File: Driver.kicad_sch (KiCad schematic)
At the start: 25 parts

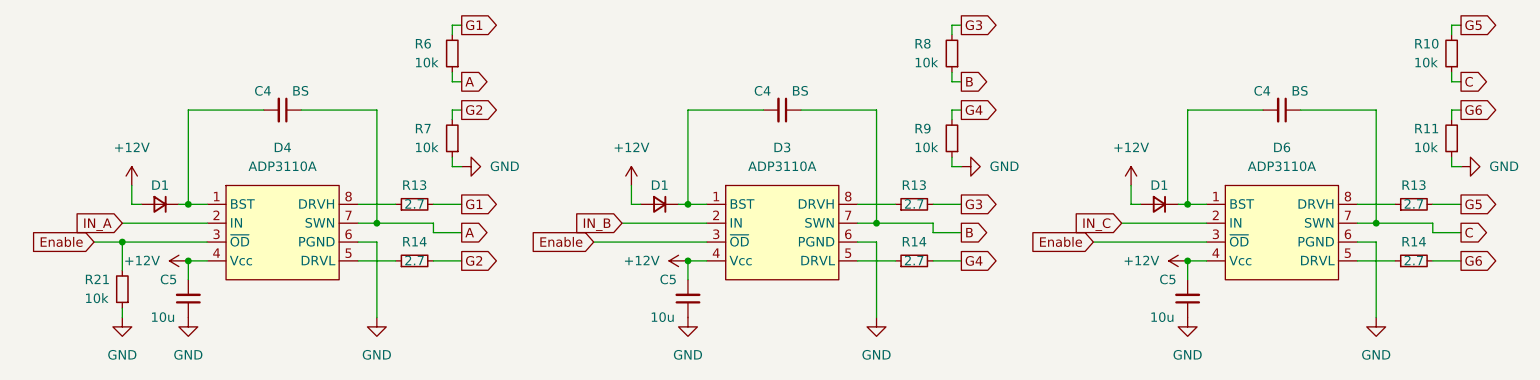
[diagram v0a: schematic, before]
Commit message: Стартовая версия
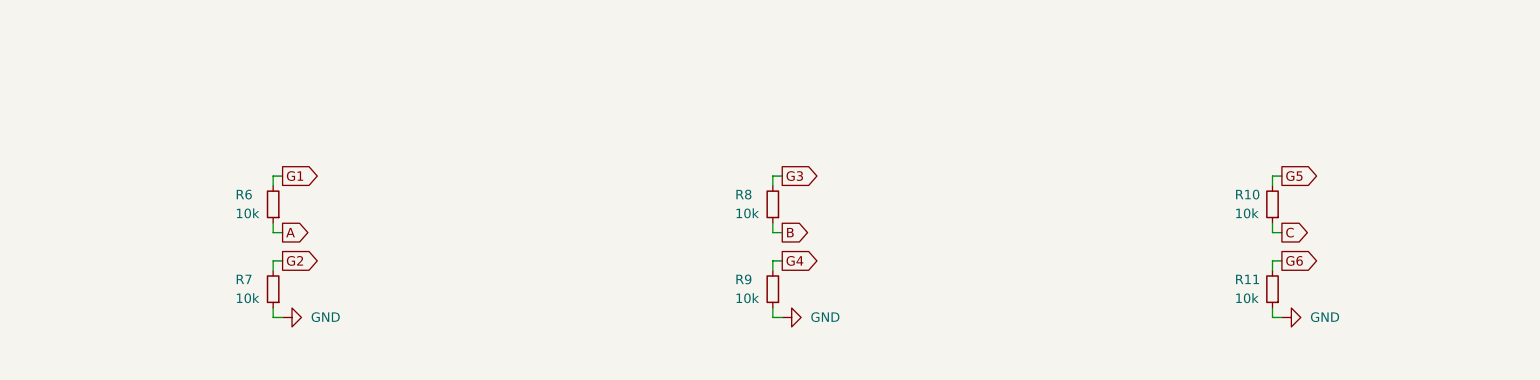
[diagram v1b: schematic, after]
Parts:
- removed C4 (x3): BS, Capacitor_SMD:C_0805_2012Metric_Pad1.18x1.45mm_HandSolder, symbol Device:C_Small
- removed C5 (x3): 10u, Capacitor_SMD:C_0805_2012Metric_Pad1.18x1.45mm_HandSolder, symbol Device:C_Small
- removed D1 (x3): D_Small, Diode_SMD:D_SOD-323, symbol Device:D_Small
- removed D3, D4, D6: ADP3110A, Package_DFN_QFN:DFN-8-1EP_3x3mm_P0.65mm_EP1.7x2.05mm, symbol IGBT_MOSFET_Drivers:ADP3110A
- removed R13 (x3), R14 (x3): 2.7, Resistor_SMD:R_0805_2012Metric_Pad1.20x1.40mm_HandSolder, symbol Device:R_Small
- removed R21: 10k, Resistor_SMD:R_0805_2012Metric_Pad1.20x1.40mm_HandSolder, symbol Device:R_Small
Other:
- moved on the sheet: R10, R11, R6, R7, R8, R9
